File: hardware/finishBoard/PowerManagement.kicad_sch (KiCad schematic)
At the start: 12 parts, among them U2 7414, U4 L78L05_SOT89

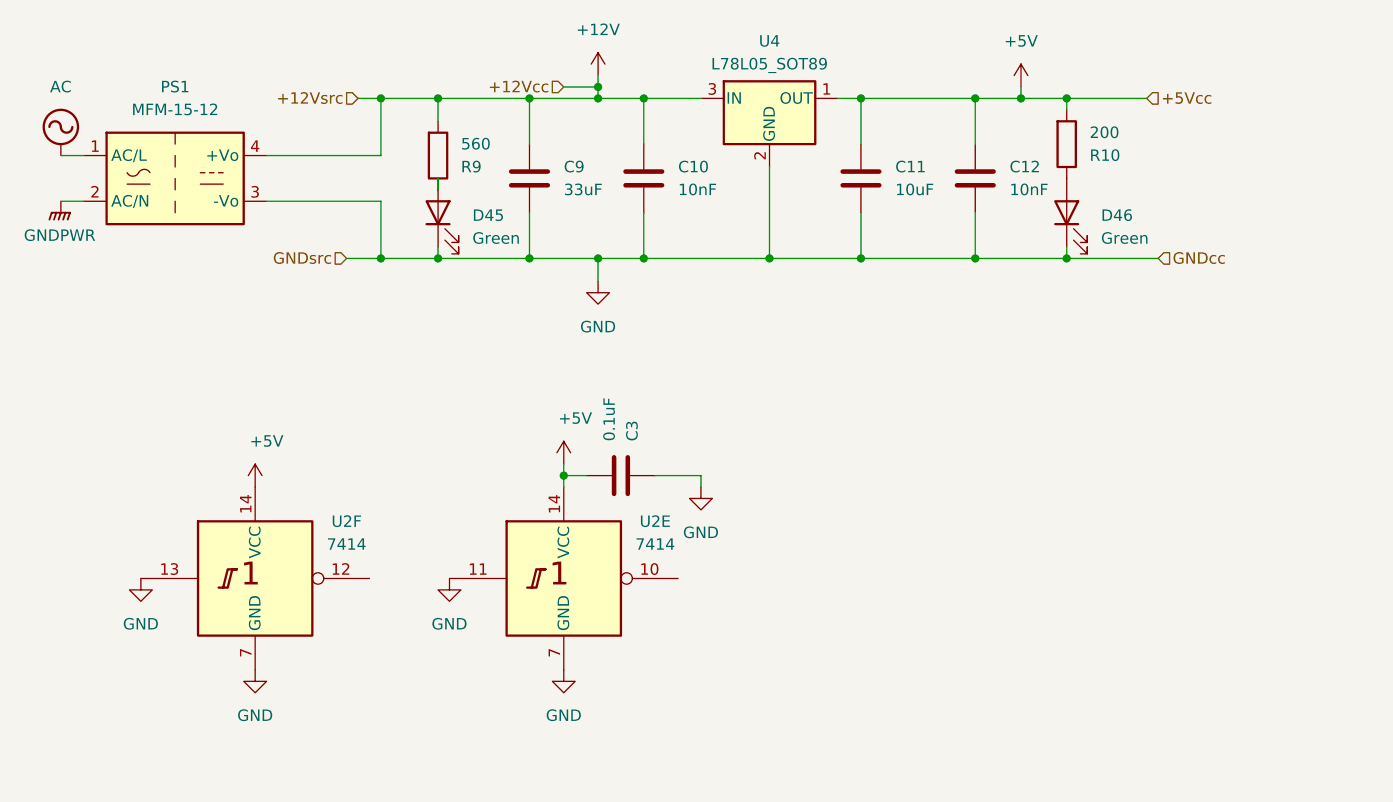
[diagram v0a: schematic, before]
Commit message: Finish Control Board completion for order
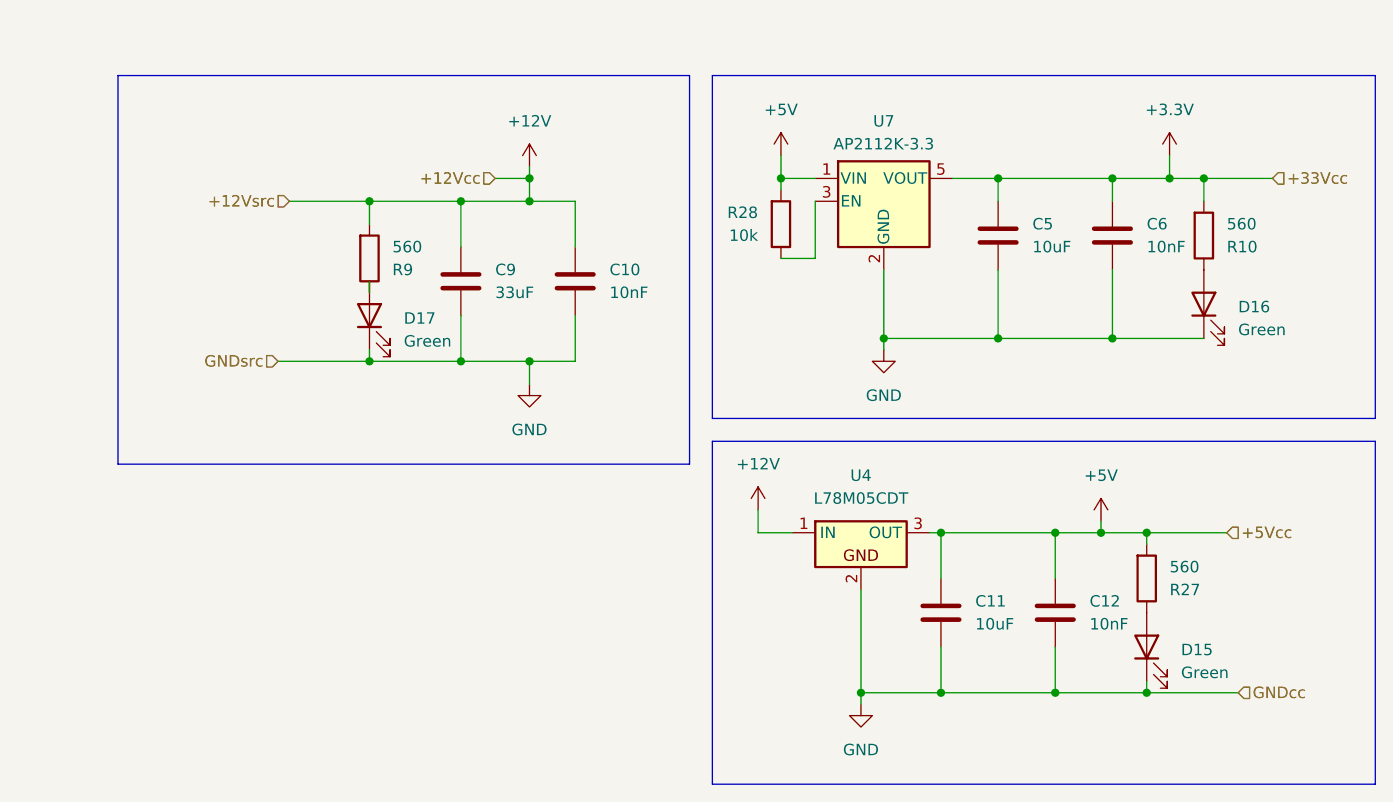
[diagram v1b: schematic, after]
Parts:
- removed C3: 0.1uF, Capacitor_SMD:C_0805_2012Metric, symbol Device:C
- removed D45, D46: Green, LED_SMD:LED_0805_2012Metric, symbol Device:LED
- removed PS1: MFM-15-12, Converter_ACDC:Converter_ACDC_MeanWell_MFM-15-xx_THT, symbol Converter_ACDC:MFM-15-12
- removed U2: 7414, Package_SO:SOIC-14_3.9x8.7mm_P1.27mm, symbol 74xx_IEEE:7414
- removed U4: L78L05_SOT89, Package_TO_SOT_SMD:SOT-89-3, symbol Regulator_Linear:L78L05_SOT89
- added C5: 10uF, Capacitor_SMD:C_0805_2012Metric, symbol Device:C
- added C6: 10nF, Capacitor_SMD:C_0805_2012Metric, symbol Device:C
- added D15, D16, D17: Green, LED_SMD:LED_0805_2012Metric_Pad1.15x1.40mm_HandSolder, symbol Device:LED
- added R27: 560, Resistor_SMD:R_0805_2012Metric, symbol Device:R
- added R28: 10k, Resistor_SMD:R_0805_2012Metric, symbol Device:R
- added U4: L78M05CDT, PCM_Package_TO_SOT_SMD_AKL:TO-252-2, symbol PCM_Voltage_Regulator_AKL:L78M05CDT
- added U7: AP2112K-3.3, Package_TO_SOT_SMD:SOT-23-5_HandSoldering, symbol Regulator_Linear:AP2112K-3.3
- R10: value 200 -> 560
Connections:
- net +12V: now also U4.1 (IN)
- net +5V: now also R27.2, R28.2, U4.3 (OUT), U7.1 (VIN); no longer R10.2
- net GND: now also C5.2, C6.2, D15.1 (K), D16.1 (K), D17.1 (K), U4.2, U7.2 (GND)
- net at R9.1: now also D17.2 (A)
- net at R10.1: now also D16.2 (A)
- new net: R28.1, U7.3 (EN)
- new net: D15.2 (A), R27.1
- new net +3.3V: C5.1, C6.1, R10.2, U7.5 (VOUT)
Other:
- moved on the sheet: C10, C11, C12, C9, R9
